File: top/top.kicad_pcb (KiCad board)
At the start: 2 copper layers, 28.8 x 40.6 mm, 23 parts, among them P1 CONN_10, P2 CONN_5, U1 IQS572, U4 ESD

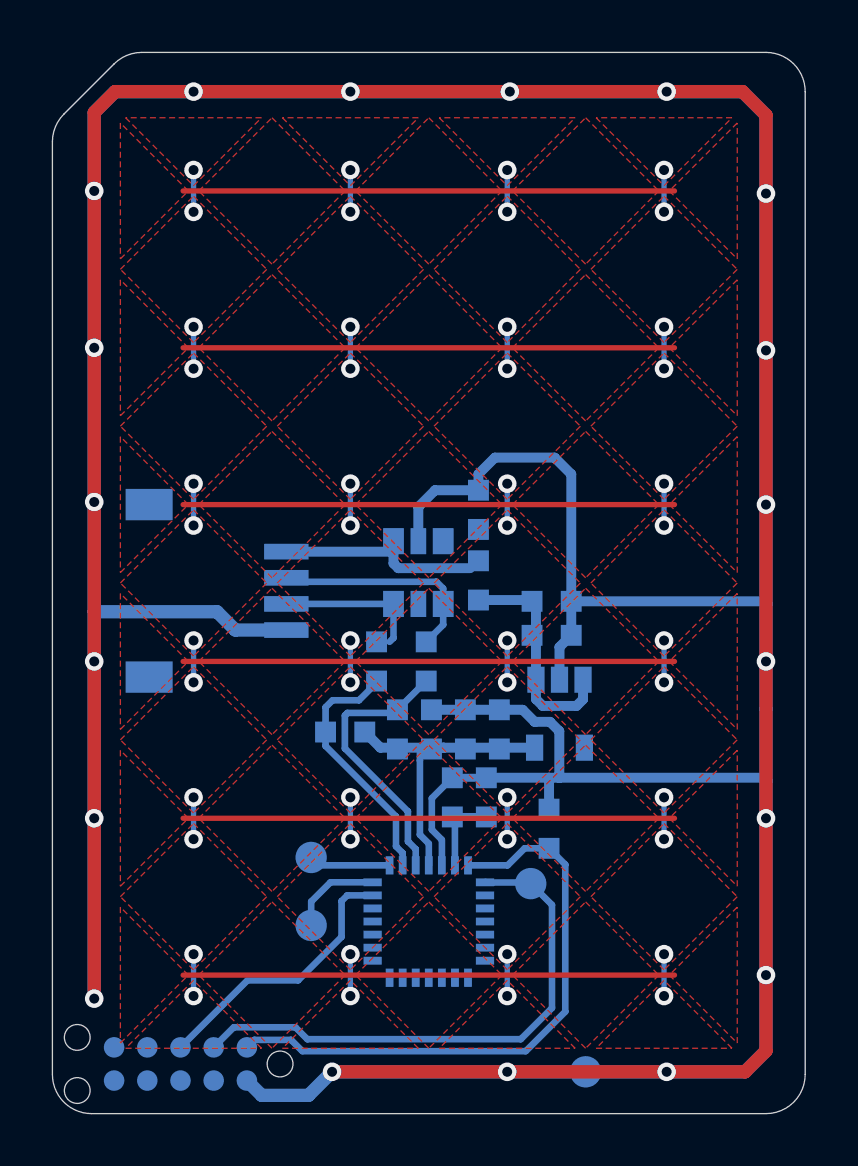
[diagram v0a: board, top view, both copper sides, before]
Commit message: First final version of PCB and SCH.
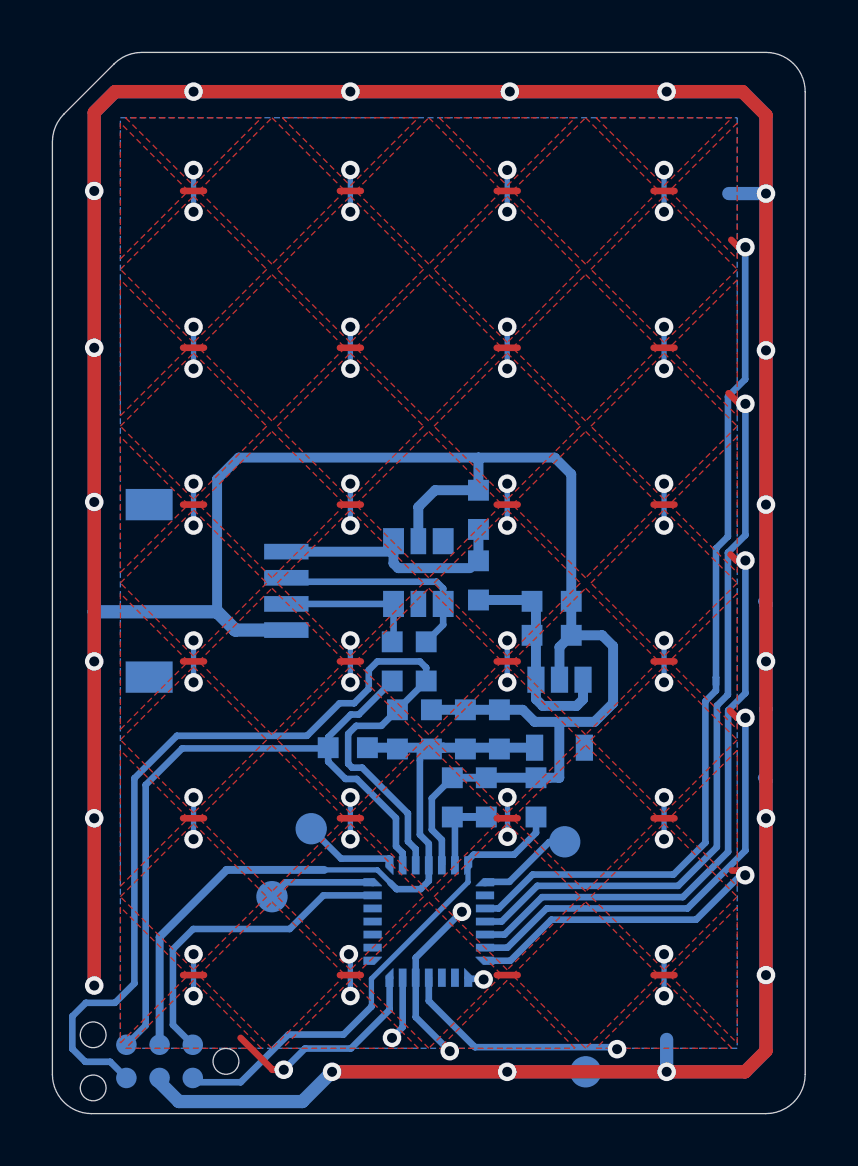
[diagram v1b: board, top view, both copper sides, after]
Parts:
- P1: value CONN_10 -> CONN_6; footprint ugl:Tag_Connect_2x5_Header_With_No_Legs -> ugl:Tag_Connect_2x3_Header_No_Legs
- U1: footprint ugl:QFN-28_4.3x4.3_Pitch0.5mm -> ugl:QFN-28_4.3x4.3_Pitch0.5mm_Alt_PAD
- moved TP_RDY1 2.06 mm to (210.9, 148.2)
- moved TP_POUT1 1.86 mm to (199.7, 150.3)
- moved C1 1.30 mm to (209.8, 146.5)
- moved TP_TOUT1 1.10 mm to (201.2, 147.7)
- moved P1 0.81 mm to (195.4, 156.6)
- moved R2 0.61 mm to (202.6, 144.6)
- moved R7 0.60 mm to (204.3, 141.3)
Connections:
- P1 pad 1: GND -> /NRST
- P1 pad 2: Net-(P1-Pad2) -> /PGM
- P1 pad 3: /SCL -> GND
- P1 pad 4: /SDA -> +3V3
- P1 pad 5: Net-(P1-Pad5) -> /SCL
- P1 pad 6: Net-(P1-Pad6) -> /SDA
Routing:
- net (no net): track 151.2 -> 0.00 mm, vias 48 -> 0
- net /RX0: track 0.00 -> 37.0 mm, vias 0 -> 1
- net /RX1: track 0.00 -> 31.5 mm, vias 0 -> 1
- net /SCL: track 10.5 -> 38.7 mm
- net /RX2: track 0.00 -> 25.9 mm, vias 0 -> 1
- net /RX3: track 0.00 -> 20.5 mm, vias 0 -> 1
- net /TX0: track 0.00 -> 18.5 mm, vias 0 -> 13
- net /TX3: track 0.00 -> 18.0 mm, vias 0 -> 13
- net /SDA: track 9.61 -> 27.5 mm
- net /RDY: track 20.8 -> 3.65 mm
- net +3V3: track 11.9 -> 28.1 mm
- net /RX4: track 0.00 -> 15.2 mm, vias 0 -> 1
- net /TX1: track 0.00 -> 14.5 mm, vias 0 -> 12
- net /TX2: track 0.00 -> 12.1 mm, vias 0 -> 13
- net GND: track 285.8 -> 296.9 mm
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- added copper zone on F.Cu, net /RX0
- added copper zone on F.Cu, net /RX1
- added copper zone on F.Cu, net /RX2
- added copper zone on F.Cu, net /RX3
- added copper zone on F.Cu, net /RX4
- added copper zone on F.Cu, net /RX5
- added copper zone on F.Cu, net /TX0
- added copper zone on F.Cu, net /TX1
- added copper zone on F.Cu, net /TX2
- added copper zone on F.Cu, net /TX3
- added copper zone on B.Cu, net GND
- removed copper zone on F.Cu, net (none)
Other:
- net class Default: clearance 0.2032 -> 0.1778
- rule trace_clearance: 0.2032 -> 0.1778
- board text added: "84981-4"
